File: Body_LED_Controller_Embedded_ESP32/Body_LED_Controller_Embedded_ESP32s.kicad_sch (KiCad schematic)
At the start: 103 parts, among them J1 SERIAL, J10 USB_B_Micro, J11 USB_B_Micro, J12 USB_B_Micro, J13 Conn_02x03_Odd_Even, J14 Conn_01x03, J15 Servo Header, J16 Screw_Terminal_01x02, J17 Screw_Terminal_01x02, J18 Screw_Terminal_01x02, J19 Screw_Terminal_01x02, J2 I2C, J20 ICSP, J21 CONSMA008, J22 U.FL-R-SMT-1(01), J3 Conn_02x10_Odd_Even, J4 LDP/MAINT, J5 COIN/VU, J6 Batt Level LEDS, J7 Data Panel/ CBI, J8 Spectrum Analyzer, J9 Ext Mic, SW1 SW_Push, SW2 SW_Push, SW3 SW_Push, U1 ATMEGA256016AU, U10 CH340C, U11 UMH3N, U12 ME6211C33M5G, U13 CJ2301_S1, U14 D36V50F5-STEPDOWN, U2 CH340C, U3 CJ2301_S1, U4 ESP32-WROOM-32U_16MB_, U5 CH340C, U6 UMH3N, U7 ME6211C33M5G, U8 CJ2301_S1, U9 ESP32-WROOM-32D_16MB_, Y1 16MHz

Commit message: Updates to some files
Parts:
- removed D1, D2: LED, LED_SMD:LED_0402_1005Metric, symbol Device:LED
- removed D3, D4, D5: APA102-2020, LED_SMD:LED-APA102-2020, symbol LED:APA102-2020
- removed J21: CONSMA008, Custom:LINX_CONSMA008, symbol Custom:CONSMA008
- removed J22: U.FL-R-SMT-1(01), Custom:HIROSE_U.FL-R-SMT-1(01), symbol Custom:U.FL-R-SMT-1(01)
- removed RN1: 10K, Custom:SOIC127P762X240-14N, symbol Device:R_Network13
- added D1, D2: SMD-LED-CLEAR-BLUE(0402), Custom:LED-0402, symbol Custom:SMD-LED-CLEAR-BLUE(0402)
- added L1, L2, L3: WS2812B-2020, WS2812B-2020, symbol LED:WS2812B-2020
- added R29, R30, R31, R32, R33, R34, R35, R36, R37, R38: 10K, Resistor_SMD:R_0402_1005Metric, symbol Device:R
- C1, C2: LCSC (none) -> C1554
- C10, C11, C4, C5, C6, C7, C8, C9: LCSC (none) -> C307331
- C12, C15, C19, C22: symbol Device:C_Polarized_Small_US -> Device:C_Small; LCSC (none) -> C315248
- C13, C14, C16, C17, C18, C20, C21, C24, C25: symbol Device:C_Polarized_Small_US -> Device:C_Small; LCSC (none) -> C307331
- C23: symbol Device:C_Polarized_Small_US -> Device:C_Small
- C3: LCSC (none) -> C315248
- CR1: LCSC (none) -> C84354
- F1: LCSC (none) -> C17313
- J1, J2, J4: LCSC (none) -> C225519
- J10, J11, J12: LCSC (none) -> C132563
- J13, J20: LCSC (none) -> C390690
- J14, J9: LCSC (none) -> C390679
- J15, J8: LCSC (none) -> C190819
- J16, J17, J18, J19: LCSC (none) -> C474892
- J3: LCSC (none) -> C492427
- J5: LCSC (none) -> C225521
- J6: LCSC (none) -> C390680
- J7: LCSC (none) -> C390682
- R1: LCSC (none) -> C328343
- R10, R11, R12, R13, R14, R26, R6, R7, R8, R9: LCSC (none) -> C352454
- R15, R16, R2, R3: LCSC (none) -> C478866
- R17: LCSC (none) -> C269701
- R18: LCSC (none) -> C245983
- R19: LCSC (none) -> C325646
- R20, R23: LCSC (none) -> C190321
- R21, R22, R24, R25: LCSC (none) -> C365065
- R4, R5: LCSC (none) -> C269674
- SW1, SW2, SW3: LCSC (none) -> C692465
- U1: LCSC (none) -> C22460
- U10, U12, U2, U5, U7: LCSC (none) -> C82942
- U11, U6: LCSC (none) -> C62892
- U13, U3, U8: LCSC (none) -> C8547
- U4: LCSC (none) -> C529580
- U9: LCSC (none) -> C529578
- Y1: LCSC (none) -> C279575
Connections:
- net +3.3V_BC: now also L2.4 (VDD)
- net +3.3V_BS: now also L1.4 (VDD)
- net +5V_BL: now also L3.4 (VDD); no longer R15.1, R16.1
- net GND: now also R15.1, R16.1, L1.2 (VSS), L2.2 (VSS), L3.2 (VSS), R29.2, R30.2, R31.2, R32.2, R33.2, R34.2, R35.2, R36.2, R37.2, R38.2
- net LIMIT1: now also R29.1
- net LIMIT10: now also R38.1
- net LIMIT2: now also R30.1
- net LIMIT3: now also R31.1
- net LIMIT4: now also R32.1
- net LIMIT5: now also R33.1
- net LIMIT6: now also R34.1
- net LIMIT7: now also R35.1
- net LIMIT8: now also R36.1
- net LIMIT9: now also R37.1
- net RXD0_BL: now also D2.+
- net TXD0_BL: now also D1.+
- net at R28.1: now also L1.3 (DI)
- net at R26.1: now also L3.3 (DI)
- net at R15.2: now also D1.-
- net at R27.1: now also L2.3 (DI)
- net at R16.2: now also D2.-
- net ST_LED_C_BC: no longer names the net of U4.31 (IO19)
- net ST_LED_C_BL: no longer names the net of U1.16 (PH4)
- net ST_LED_C_BS: no longer names the net of U9.31 (IO19)
- no-connect marks 123 -> 122
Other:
- moved on the sheet: R26, R27, R28

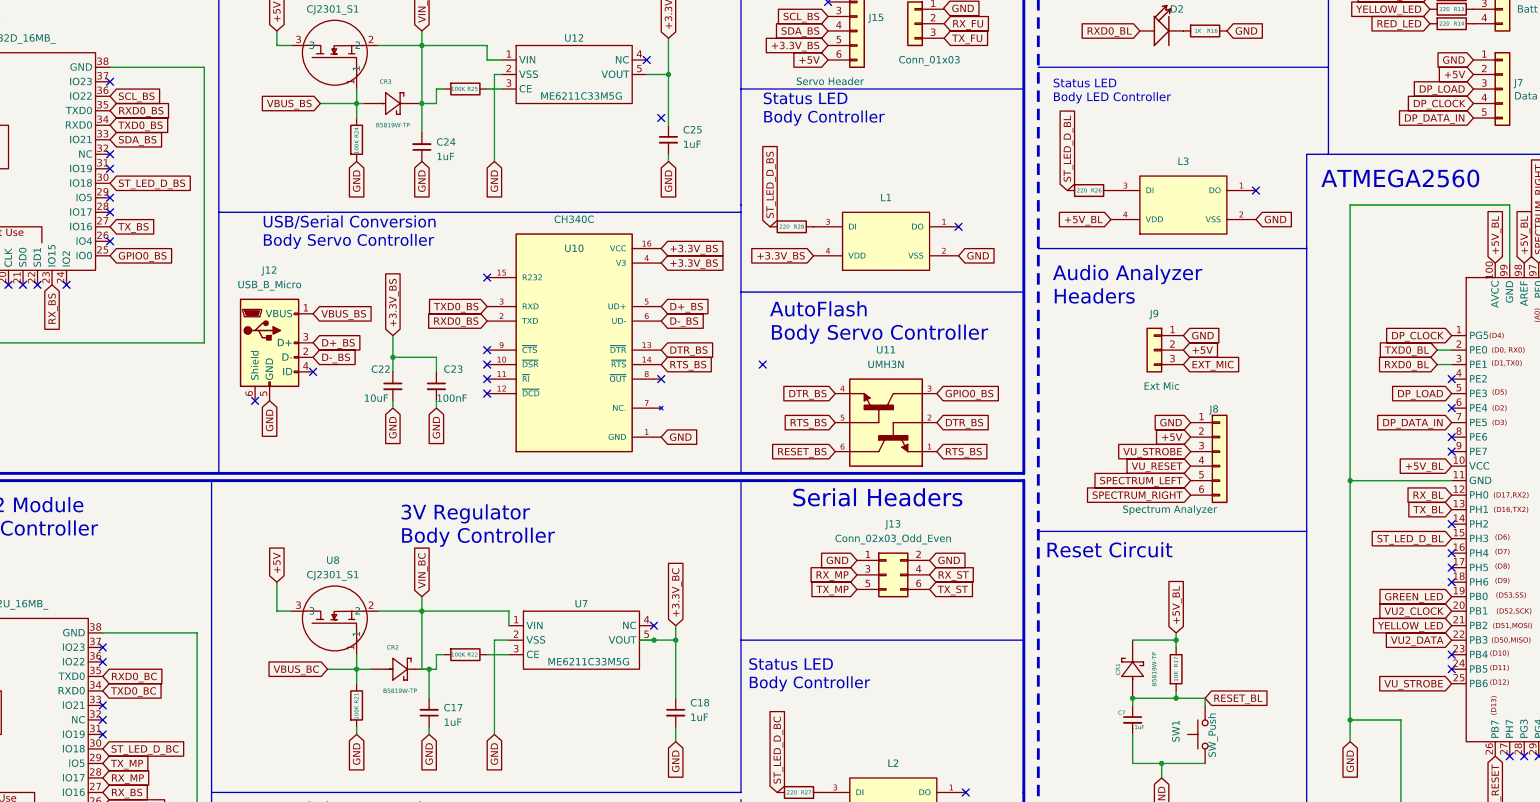
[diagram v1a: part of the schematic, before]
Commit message: updates to the boards
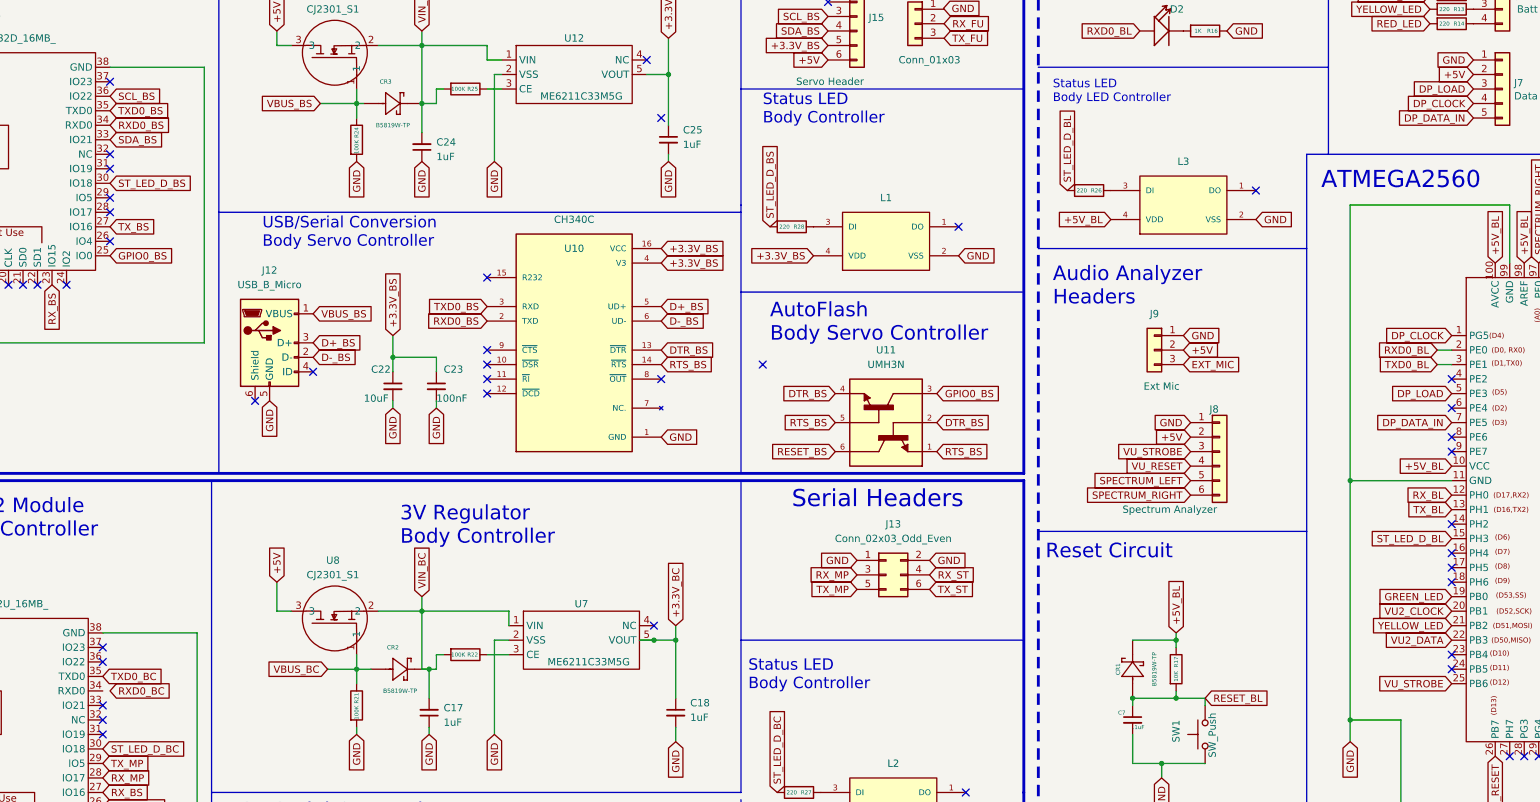
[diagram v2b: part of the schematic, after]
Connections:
- net RXD0_BC: no longer U4.35 (TXD0)
- net RXD0_BL: now also U1.2 (PE0); no longer U1.3 (PE1)
- net RXD0_BS: now also U9.34 (RXD0); no longer U9.35 (TXD0)
- net TXD0_BC: now also U4.35 (TXD0); no longer U4.34 (RXD0)
- net TXD0_BL: now also U1.3 (PE1); no longer U1.2 (PE0)
- net TXD0_BS: now also U9.35 (TXD0); no longer U9.34 (RXD0)
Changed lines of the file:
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@@
     )
   )
-  (global_label "TXD0_BS" (shape input) (at 88.9 104.14 0) (fields_autoplaced)
-    (effects (font (size 1.27 1.27)) (justify left))
-    (property "Intersheet References" "${INTERSHEET_REFS}" (id 0) (at 99.328 104.2194 0)
+  (global_label "TXD0_BS" (shape input) (at 88.9 101.6 0) (fields_autoplaced)
+    (effects (font (size 1.27 1.27)) (justify left))
+    (property "Intersheet References" "${INTERSHEET_REFS}" (id 0) (at 99.328 101.6794 0)
       (effects (font (size 1.27 1.27)) (justify left) hide)
     )
@@
     )
   )
-  (global_label "RXD0_BS" (shape input) (at 88.9 101.6 0) (fields_autoplaced)
-    (effects (font (size 1.27 1.27)) (justify left))
-    (property "Intersheet References" "${INTERSHEET_REFS}" (id 0) (at 99.6304 101.6794 0)
-      (effects (font (size 1.27 1.27)) (justify left) hide)
-    )
-  )
-  (global_label "RXD0_BC" (shape input) (at 87.63 200.66 0) (fields_autoplaced)
-    (effects (font (size 1.27 1.27)) (justify left))
-    (property "Intersheet References" "${INTERSHEET_REFS}" (id 0) (at 98.4209 200.7394 0)
+  (global_label "RXD0_BS" (shape input) (at 88.9 104.14 0) (fields_autoplaced)
+    (effects (font (size 1.27 1.27)) (justify left))
+    (property "Intersheet References" "${INTERSHEET_REFS}" (id 0) (at 99.6304 104.2194 0)
+      (effects (font (size 1.27 1.27)) (justify left) hide)
+    )
+  )
+  (global_label "RXD0_BC" (shape input) (at 88.9 203.2 0) (fields_autoplaced)
+    (effects (font (size 1.27 1.27)) (justify left))
+    (property "Intersheet References" "${INTERSHEET_REFS}" (id 0) (at 99.6909 203.2794 0)
       (effects (font (size 1.27 1.27)) (justify left) hide)
     )
@@
     )
   )
-  (global_label "RXD0_BL" (shape input) (at 321.31 146.05 180) (fields_autoplaced)
-    (effects (font (size 1.27 1.27)) (justify right))
-    (property "Intersheet References" "${INTERSHEET_REFS}" (id 0) (at 310.761 145.9706 0)
+  (global_label "RXD0_BL" (shape input) (at 321.31 143.51 180) (fields_autoplaced)
+    (effects (font (size 1.27 1.27)) (justify right))
+    (property "Intersheet References" "${INTERSHEET_REFS}" (id 0) (at 310.761 143.4306 0)
       (effects (font (size 1.27 1.27)) (justify right) hide)
     )
@@
     )
   )
-  (global_label "TXD0_BC" (shape input) (at 87.63 203.2 0) (fields_autoplaced)
-    (effects (font (size 1.27 1.27)) (justify left))
-    (property "Intersheet References" "${INTERSHEET_REFS}" (id 0) (at 98.1185 203.2794 0)
+  (global_label "TXD0_BC" (shape input) (at 87.63 200.66 0) (fields_autoplaced)
+    (effects (font (size 1.27 1.27)) (justify left))
+    (property "Intersheet References" "${INTERSHEET_REFS}" (id 0) (at 98.1185 200.7394 0)
       (effects (font (size 1.27 1.27)) (justify left) hide)
     )
@@
     )
   )
-  (global_label "TXD0_BL" (shape input) (at 321.31 143.51 180) (fields_autoplaced)
-    (effects (font (size 1.27 1.27)) (justify right))
-    (property "Intersheet References" "${INTERSHEET_REFS}" (id 0) (at 311.0634 143.4306 0)
-      (effects (font (size 1.27 1.27)) (justify right) hide)
-    )
+  (global_label "TXD0_BL" (shape input) (at 321.31 146.05 180) (fields_autoplaced)
+    (effects (font (size 1.27 1.27)) (justify right))
+    (property "Intersheet References" "${INTERSHEET_REFS}" (id 0) (at 311.0634 145.9706 0)
+      (effects (font (size 1.27 1.27)) (justify right) hide)
+    )
